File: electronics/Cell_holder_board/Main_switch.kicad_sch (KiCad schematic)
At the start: 7 parts, among them Q1 IRLB8721PBF, Q2 IRLB8721PBF, U1 LTV-817

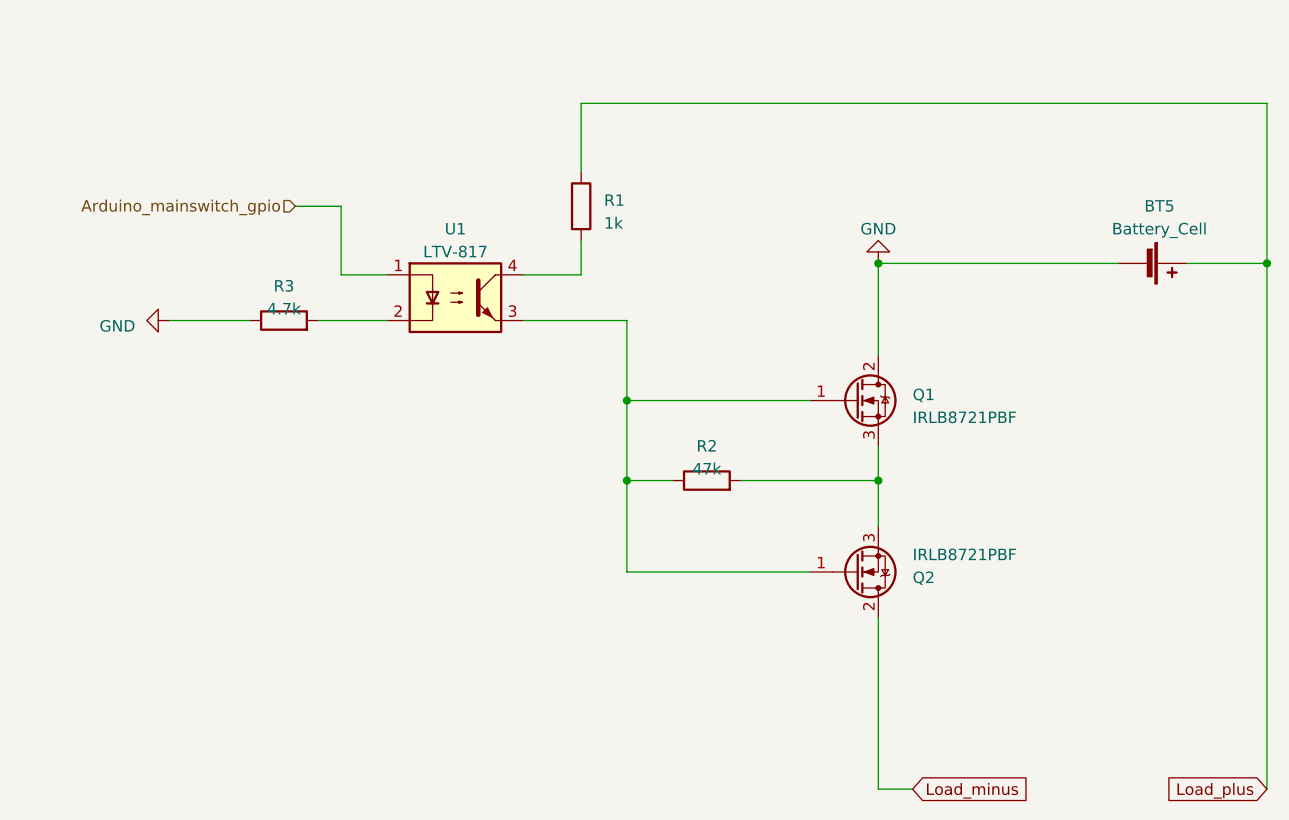
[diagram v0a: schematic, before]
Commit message: discord session with Johannes and Fabian, Schematic nearly done, all footprints fields filled
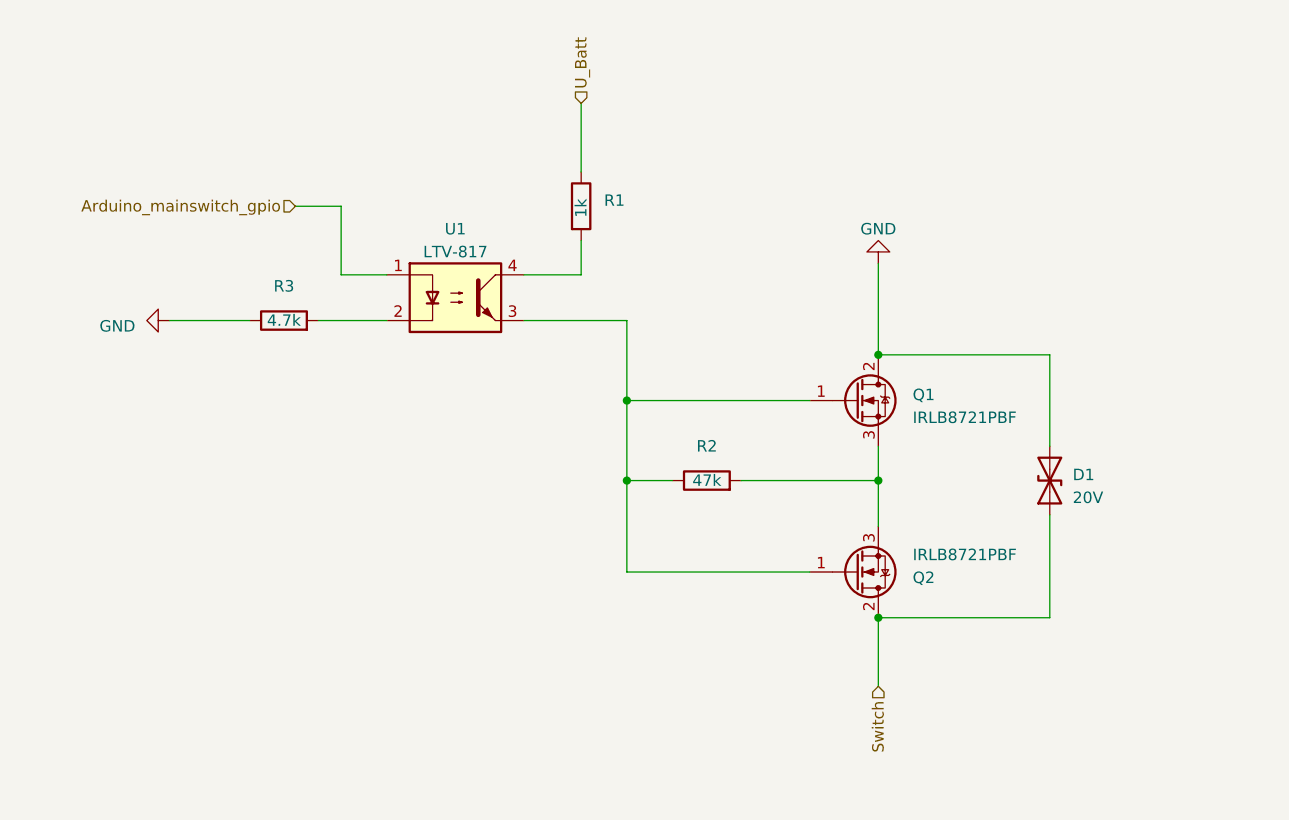
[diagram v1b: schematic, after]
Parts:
- removed BT5: Battery_Cell, symbol Device:Battery_Cell
- added D1: 20V, Diode_SMD:D_SMA, symbol Device:D_TVS
- R1, R2, R3: footprint (none) -> Resistor_SMD:R_0805_2012Metric
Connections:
- net GND: now also D1.2 (A2)
- net Load_minus renamed Switch
- net Switch: now also D1.1 (A1)
- net Load_plus renamed U_Batt
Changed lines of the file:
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@@
 (kicad_sch (version 20230121) (generator eeschema)
   (paper "A4")
-  (junction (at 139.7 54.61) (diameter 0) (color 0 0 0 0)
-  )
   (junction (at 111.76 69.85) (diameter 0) (color 0 0 0 0)
   )
-  (junction (at 182.88 54.61) (diameter 0) (color 0 0 0 0)
+  (junction (at 139.7 93.98) (diameter 0) (color 0 0 0 0)
   )
   (junction (at 111.76 78.74) (diameter 0) (color 0 0 0 0)
   )
+  (junction (at 139.7 64.77) (diameter 0) (color 0 0 0 0)
+  )
   (junction (at 139.7 78.74) (diameter 0) (color 0 0 0 0)
   )
-  (wire (pts (xy 139.7 93.98) (xy 139.7 113.03))
-    (stroke (width 0) (type default))
-  )
   (wire (pts (xy 111.76 69.85) (xy 111.76 60.96))
     (stroke (width 0) (type default))
@@
     (stroke (width 0) (type default))
   )
+  (wire (pts (xy 158.75 93.98) (xy 139.7 93.98))
+    (stroke (width 0) (type default))
+  )
   (wire (pts (xy 139.7 78.74) (xy 139.7 83.82))
     (stroke (width 0) (type default))
@@
     (stroke (width 0) (type default))
   )
-  (wire (pts (xy 182.88 54.61) (xy 182.88 36.83))
+  (wire (pts (xy 158.75 74.93) (xy 158.75 64.77))
     (stroke (width 0) (type default))
   )
@@
     (stroke (width 0) (type default))
   )
+  (wire (pts (xy 139.7 93.98) (xy 139.7 101.6))
+    (stroke (width 0) (type default))
+  )
   (wire (pts (xy 111.76 78.74) (xy 111.76 88.9))
     (stroke (width 0) (type default))
   )
-  (wire (pts (xy 182.88 54.61) (xy 182.88 113.03))
-    (stroke (width 0) (type default))
-  )
   (wire (pts (xy 132.08 69.85) (xy 111.76 69.85))
     (stroke (width 0) (type default))
@@
     (stroke (width 0) (type default))
   )
-  (wire (pts (xy 166.37 54.61) (xy 139.7 54.61))
-    (stroke (width 0) (type default))
-  )
   (wire (pts (xy 106.68 36.83) (xy 106.68 44.45))
     (stroke (width 0) (type default))
   )
-  (wire (pts (xy 173.99 54.61) (xy 182.88 54.61))
-    (stroke (width 0) (type default))
-  )
   (wire (pts (xy 139.7 54.61) (xy 139.7 64.77))
     (stroke (width 0) (type default))
   )
-  (wire (pts (xy 139.7 113.03) (xy 143.51 113.03))
-    (stroke (width 0) (type default))
-  )
   (wire (pts (xy 111.76 88.9) (xy 132.08 88.9))
     (stroke (width 0) (type default))
   )
-  (wire (pts (xy 106.68 36.83) (xy 182.88 36.83))
-    (stroke (width 0) (type default))
-  )
   (wire (pts (xy 111.76 69.85) (xy 111.76 78.74))
     (stroke (width 0) (type default))
@@
     (stroke (width 0) (type default))
   )
+  (wire (pts (xy 158.75 64.77) (xy 139.7 64.77))
+    (stroke (width 0) (type default))
+  )
+  (wire (pts (xy 158.75 82.55) (xy 158.75 93.98))
+    (stroke (width 0) (type default))
+  )
   (wire (pts (xy 124.46 78.74) (xy 139.7 78.74))
     (stroke (width 0) (type default))
@@
     (stroke (width 0) (type default))
   )
-  (global_label "Load_minus" (shape input) (at 143.51 113.03 0) (fields_autoplaced)
-    (effects (font (size 1.27 1.27)) (justify left))
-    (property "Intersheetrefs" "${INTERSHEET_REFS}" (at 157.4827 113.03 0)
-      (effects (font (size 1.27 1.27)) (justify left) hide)
-    )
-  )
-  (global_label "Load_plus" (shape input) (at 182.88 113.03 180) (fields_autoplaced)
+  (hierarchical_label "Switch" (shape input) (at 139.7 101.6 270) (fields_autoplaced)
     (effects (font (size 1.27 1.27)) (justify right))
-    (property "Intersheetrefs" "${INTERSHEET_REFS}" (at 170.5402 113.03 0)
-      (effects (font (size 1.27 1.27)) (justify right) hide)
-    )
   )
   (hierarchical_label "Arduino_mainswitch_gpio" (shape input) (at 74.93 48.26 180) (fields_autoplaced)
     (effects (font (size 1.27 1.27)) (justify right))
   )
+  (hierarchical_label "U_Batt" (shape input) (at 106.68 36.83 90) (fields_autoplaced)
+    (effects (font (size 1.27 1.27)) (justify left))
+  )
   (symbol (lib_id "Device:R") (at 120.65 78.74 90) (unit 1)
-    (in_bom yes) (on_board yes) (dnp no) (fields_autoplaced)
+    (in_bom yes) (on_board yes) (dnp no)
     (property "Reference" "R2" (at 120.65 74.93 90)
       (effects (font (size 1.27 1.27)))
     )
-    (property "Value" "47k" (at 120.65 77.47 90)
-      (effects (font (size 1.27 1.27)))
-    )
-    (property "Footprint" "" (at 120.65 80.518 90)
+    (property "Value" "47k" (at 120.65 78.74 90)
+      (effects (font (size 1.27 1.27)))
+    )
+    (property "Footprint" "Resistor_SMD:R_0805_2012Metric" (at 120.65 80.518 90)
       (effects (font (size 1.27 1.27)) hide)
     )
@@
         (path "/c2697d40-f04f-4888-9ae9-ce0b7f222632/58237fb8-3152-4ac3-938c-94583c912e78"
           (reference "R2") (unit 1)
+        )
+      )
+    )
+  )
+  (symbol (lib_id "Device:D_TVS") (at 158.75 78.74 90) (unit 1)
+    (in_bom yes) (on_board yes) (dnp no) (fields_autoplaced)
+    (property "Reference" "D1" (at 161.29 78.105 90)
+      (effects (font (size 1.27 1.27)) (justify right))
+    )
+    (property "Value" "20V" (at 161.29 80.645 90)
+      (effects (font (size 1.27 1.27)) (justify right))
+    )
+    (property "Footprint" "Diode_SMD:D_SMA" (at 158.75 78.74 0)
+      (effects (font (size 1.27 1.27)) hide)
+    )
+    (property "Datasheet" "~" (at 158.75 78.74 0)
+      (effects (font (size 1.27 1.27)) hide)
+    )
+    (pin "1")
+    (pin "2")
+    (instances
+      (project "Cell_holder_board"
+        (path "/c2697d40-f04f-4888-9ae9-ce0b7f222632/58237fb8-3152-4ac3-938c-94583c912e78"
+          (reference "D1") (unit 1)
         )
       )
@@
     )
   )
-  (symbol (lib_id "Device:Battery_Cell") (at 168.91 54.61 270) (unit 1)
-    (in_bom yes) (on_board yes) (dnp no) (fields_autoplaced)
-    (property "Reference" "BT5" (at 170.942 48.26 90)
-      (effects (font (size 1.27 1.27)))
-    )
-    (property "Value" "Battery_Cell" (at 170.942 50.8 90)
-      (effects (font (size 1.27 1.27)))
-    )
-    (property "Footprint" "" (at 170.434 54.61 90)
-      (effects (font (size 1.27 1.27)) hide)
-    )
-    (property "Datasheet" "~" (at 170.434 54.61 90)
-      (effects (font (size 1.27 1.27)) hide)
-    )
-    (pin "1")
-    (pin "2")
-    (instances
-      (project "Cell_holder_board"
-        (path "/c2697d40-f04f-4888-9ae9-ce0b7f222632/58237fb8-3152-4ac3-938c-94583c912e78"
-          (reference "BT5") (unit 1)
-        )
-      )
-    )
-  )
   (symbol (lib_id "Isolator:LTV-817") (at 92.71 58.42 0) (unit 1)
     (in_bom yes) (on_board yes) (dnp no) (fields_autoplaced)
@@
   )
   (symbol (lib_id "Device:R") (at 73.66 60.96 90) (unit 1)
-    (in_bom yes) (on_board yes) (dnp no) (fields_autoplaced)
+    (in_bom yes) (on_board yes) (dnp no)
     (property "Reference" "R3" (at 73.66 57.15 90)
       (effects (font (size 1.27 1.27)))
     )
-    (property "Value" "4.7k" (at 73.66 59.69 90)
-      (effects (font (size 1.27 1.27)))
-    )
-    (property "Footprint" "" (at 73.66 62.738 90)
+    (property "Value" "4.7k" (at 73.66 60.96 90)
+      (effects (font (size 1.27 1.27)))
+    )
+    (property "Footprint" "Resistor_SMD:R_0805_2012Metric" (at 73.66 62.738 90)
       (effects (font (size 1.27 1.27)) hide)
     )
@@
   )
   (symbol (lib_id "Device:R") (at 106.68 48.26 0) (unit 1)
-    (in_bom yes) (on_board yes) (dnp no) (fields_autoplaced)
+    (in_bom yes) (on_board yes) (dnp no)
     (property "Reference" "R1" (at 109.22 47.625 0)
       (effects (font (size 1.27 1.27)) (justify left))
     )
-    (property "Value" "1k" (at 109.22 50.165 0)
-      (effects (font (size 1.27 1.27)) (justify left))
-    )
-    (property "Footprint" "" (at 104.902 48.26 90)
-      (effects (font (size 1.27 1.27)) hide)
-    )
+    (property "Value" "1k" (at 106.68 49.53 90)
+      (effects (font (size 1.27 1.27)) (justify left))
+    )
+    (property "Footprint" "Resistor_SMD:R_0805_2012Metric" (at 104.902 48.26 90)
+      (effects (font (size 1.27 1.27)) hide)
+    )
